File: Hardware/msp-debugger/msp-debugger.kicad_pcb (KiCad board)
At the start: 2 copper layers, 195.6 x 98 mm, 22 parts, among them J1 USB_B_Micro, J2 Conn_02x10, J3 Conn_02x10, J4 Conn_01x04_Pin, SW1 222ADVBA, SW2 222ADVBA, SW3 222ADVBA, SW4 222ADVBA, SW5 222ADVBA, U1 MSP430G2553IN20, U3 BA033CC0FP-E2, U4 FT230XS-R

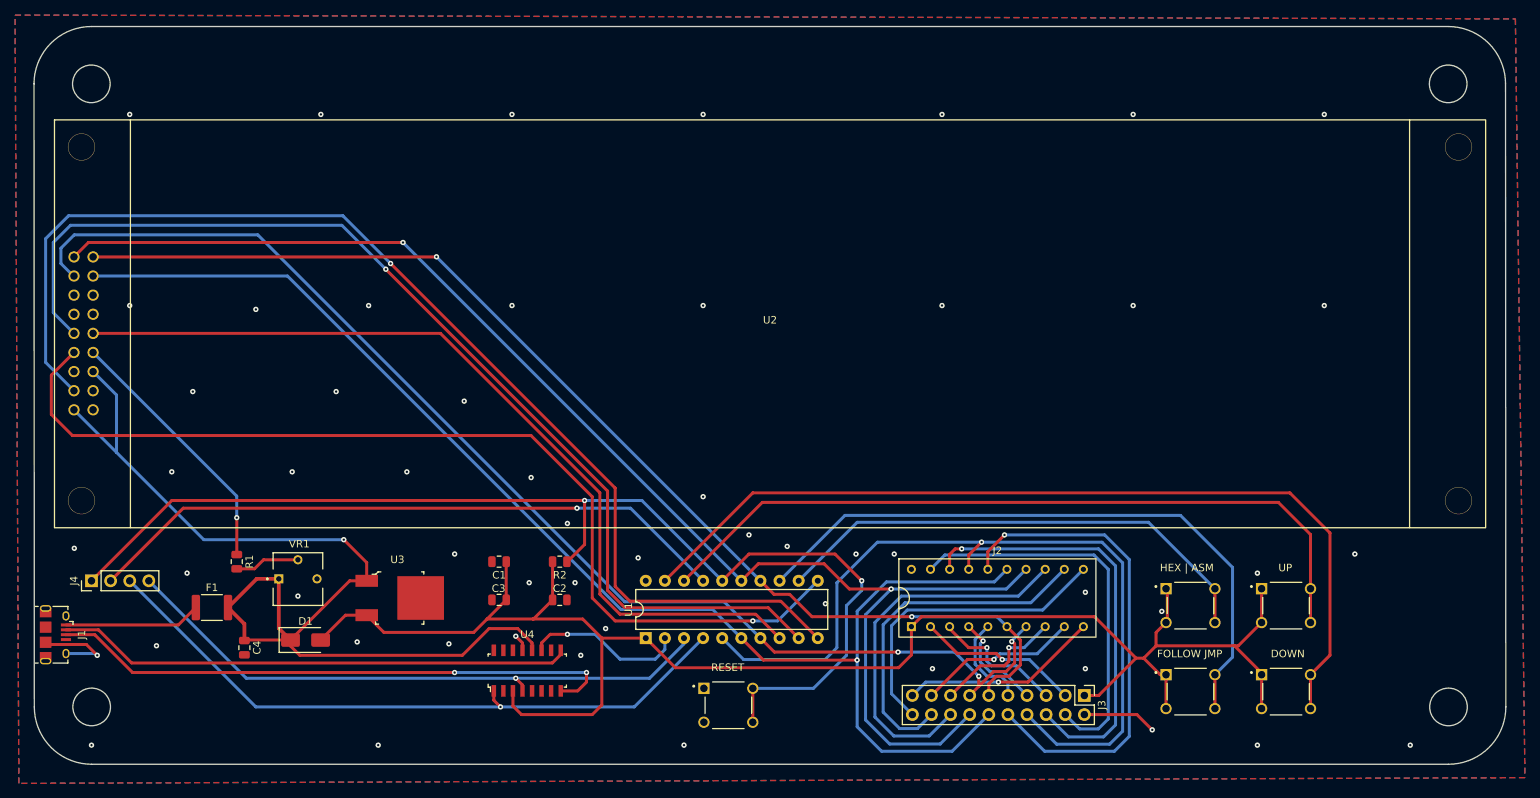
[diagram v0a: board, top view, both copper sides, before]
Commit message: fix hardware issues and route small pcb
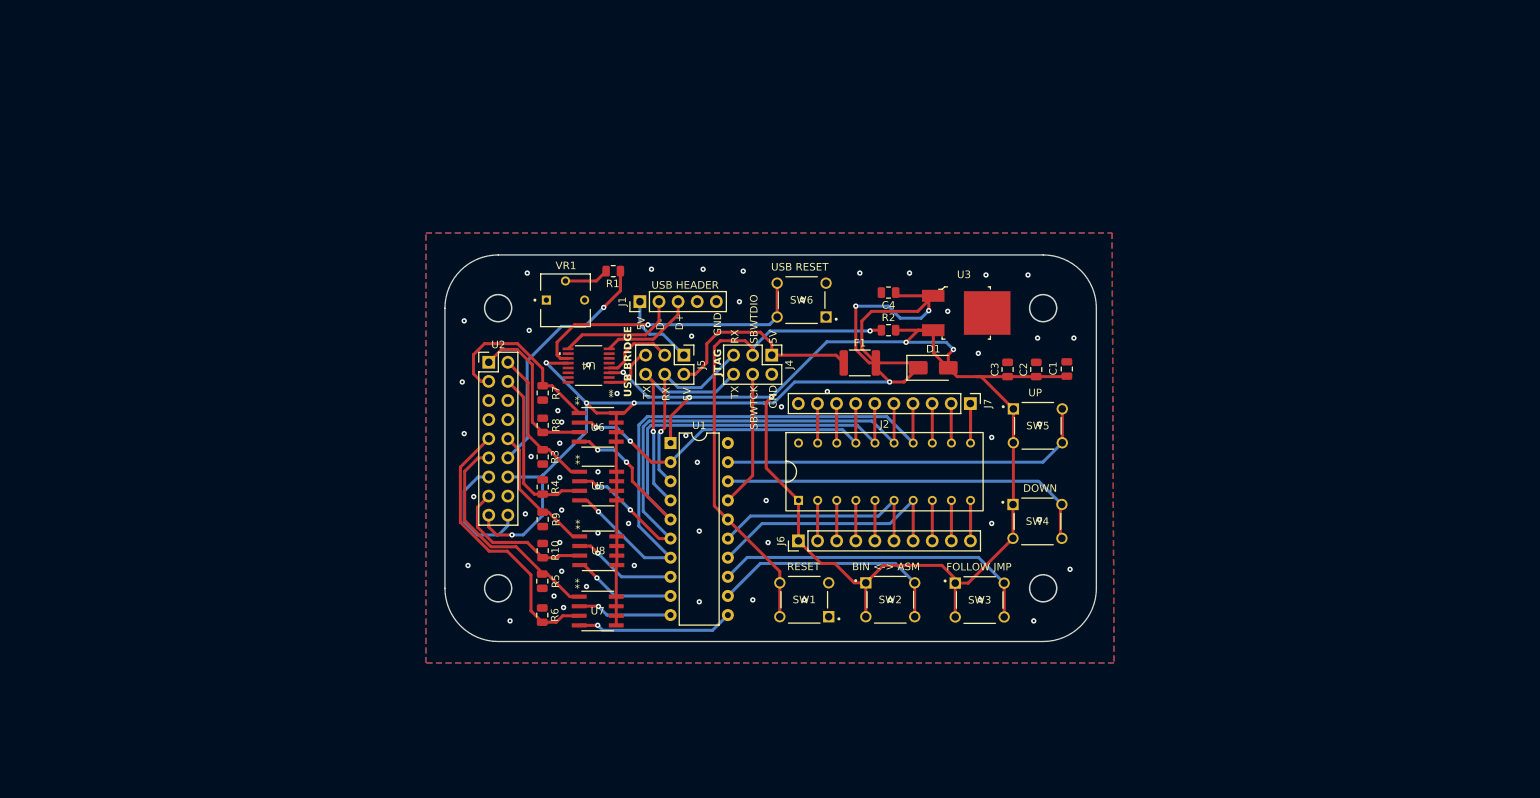
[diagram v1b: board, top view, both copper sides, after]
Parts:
- removed J3: Conn_02x10, Connector_PinHeader_2.54mm:PinHeader_2x10_P2.54mm_Vertical
- added J5: USB JUMPER, Connector_PinHeader_2.54mm:PinHeader_2x03_P2.54mm_Vertical, F.Cu at (137.1, 82.8)
- added J6: Conn_01x10, Connector_PinHeader_2.54mm:PinHeader_1x10_P2.54mm_Vertical, F.Cu at (152.4, 107.5)
- added J7: Conn_01x10, Connector_PinHeader_2.54mm:PinHeader_1x10_P2.54mm_Vertical, F.Cu at (175.2, 89.2)
- added R10: 10K, Capacitor_SMD:C_0805_2012Metric, F.Cu at (118.4, 108.8)
- added R3: 10K, Capacitor_SMD:C_0805_2012Metric, F.Cu at (118.4, 96.3)
- added R4: 10K, Capacitor_SMD:C_0805_2012Metric, F.Cu at (118.4, 100.3)
- added R5: 10K, Capacitor_SMD:C_0805_2012Metric, F.Cu at (118.3, 112.8)
- added R6: 10K, Capacitor_SMD:C_0805_2012Metric, F.Cu at (118.3, 117.3)
- added R7: 10K, Capacitor_SMD:C_0805_2012Metric, F.Cu at (118.4, 87.8)
- added R8: 10K, Capacitor_SMD:C_0805_2012Metric, F.Cu at (118.4, 92.1)
- added R9: 10K, Capacitor_SMD:C_0805_2012Metric, F.Cu at (118.4, 104.6)
- added SW6: 222ADVBA, buttons:SW_222ADVBA, F.Cu at (152.8, 75.5)
- added U5: AO4882, project:SO-8_AOS, F.Cu at (125.7, 100.2)
- added U6: AO4882, project:SO-8_AOS, F.Cu at (125.7, 92.4)
- added U7: AO4882, project:SO-8_AOS, F.Cu at (125.7, 116.8)
- added U8: AO4882, project:SO-8_AOS, F.Cu at (125.8, 108.8)
- J1: footprint Connector_USB:USB_Micro-B_Amphenol_10118194_Horizontal -> Connector_PinHeader_2.54mm:PinHeader_1x05_P2.54mm_Vertical
- J4: value Conn_01x04_Pin -> MSP_FET PORT; footprint Connector_PinHeader_2.54mm:PinHeader_1x04_P2.54mm_Vertical -> Connector_PinHeader_2.54mm:PinHeader_2x03_P2.54mm_Vertical
- U2: footprint project:NHD-0440AZ-FL-YBW -> Connector_PinHeader_2.54mm:PinHeader_2x09_P2.54mm_Vertical
- U4: footprint digikey-footprints:SOIC-16_W3.90mm -> project:SOIC_30XS-R_FTD
- moved C4 97.7 mm to (164.3, 74.5), turned to 180 degrees
- moved J4 95.3 mm to (148.8, 82.8), turned to -90 degrees
- moved F1 92.0 mm to (160.5, 83.8)
- moved D1 90.9 mm to (170.3, 84.5)
- moved J1 89.4 mm to (131.3, 75.7), turned to 90 degrees
- moved U3 84.3 mm to (174.4, 77.2)
- moved C1 79.7 mm to (188.0, 84.6), turned to -90 degrees
- moved C3 74.2 mm to (180.2, 84.7), turned to 90 degrees
- moved C2 70.3 mm to (184.0, 84.7), turned to 90 degrees
- moved R1 63.2 mm to (127.8, 71.6), turned to 180 degrees
- moved R2 53.4 mm to (164.3, 79.5), turned to 0 degrees
- moved VR1 51.4 mm to (121.4, 75.5)
- moved U4 41.4 mm to (124.5, 84.2), turned to 180 degrees
- moved SW5 40.7 mm to (184.2, 92.2)
- moved SW4 40.0 mm to (184.1, 104.9)
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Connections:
- F1 pad 1: Net-(J1-VBUS) -> /PWR_IN
- J1 pad 1: Net-(J1-VBUS) -> /USB_IN
- J2 pad 14: /DB7 -> /DB4
- J2 pad 15: /DB4 -> /DB6
- J2 pad 16: /RST -> /DB7
- J2 pad 17: /TEST -> /DB5
- J2 pad 6: /DB6 -> /TCK
- J2 pad 7: /DB5 -> /TMS
- J4 pad 1: /CNTL RST -> /PWR_IN
- J4 pad 2: /SBWTCK -> GND
- J4 pad 3: /BC_TX -> /CNTL RST
- J4 pad 4: /BC_RX -> /SBWTCK
- U1 pad 10: /E2 -> /RS
- U1 pad 11: /RS -> /E1
- U1 pad 14: /DB6 -> /TMS
- U1 pad 15: /DB7 -> /TCK
- U1 pad 18: /UP SW -> /DOWN SW
- U1 pad 19: /DOWN SW -> /UP SW
- U1 pad 2: /RESET# -> /DB5
- U1 pad 5: /TEST -> /DB7
- U1 pad 6: /DB4 -> /DB6
- U1 pad 7: /DB5 -> /DB4
- U1 pad 9: /E1 -> /E2
- U2 pad 1: /DB7 -> /DB7_5V
- U2 pad 10: /R/W -> /R/W_5V
- U2 pad 11: /RS -> /RS_5V
- U2 pad 15: /E2 -> /E2_5V
- U2 pad 2: /DB6 -> /DB6_5V
- U2 pad 3: /DB5 -> /DB5_5V
- U2 pad 4: /DB4 -> /DB4_5V
- U2 pad 9: /E1 -> /E1_5V
- U4 pad 1: /BC_TX -> /BRIDGE_TX
- U4 pad 4: /BC_RX -> /BRIDGE_RX
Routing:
- net /E2: track 156.6 -> 13.8 mm
- net /E1: track 143.7 -> 20.9 mm
- net /RS: track 132.8 -> 12.6 mm
- net /DB5: track 166.4 -> 46.7 mm, vias 3 -> 2
- net /DB7: track 184.9 -> 67.4 mm
- net /TEST: track 108.8 -> 0.00 mm, vias 1 -> 0
- net /DB4: track 181.1 -> 78.3 mm
- net /R/W: track 115.9 -> 13.8 mm, vias 0 -> 1
- net /CNTL RST: track 152.8 -> 65.2 mm, vias 2 -> 1
- net /DB6: track 154.4 -> 71.7 mm
- net /DOWN SW: track 119.8 -> 50.2 mm
- net /SBWTCK: track 86.7 -> 18.1 mm, vias 1 -> 0
- net /RST: track 65.9 -> 0.00 mm, vias 1 -> 0
- net /D+: track 76.4 -> 12.8 mm, vias 2 -> 0
- net /BC_TX: track 89.4 -> 31.8 mm
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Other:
- board size 195.6 x 98 mm -> 86.6 x 51.4 mm
- board text added: "5V"
- board text added: "D+"
- board text added: "D-"
- board text added: "GND"
- board text added: "JTAG"
- board text added: "RX"
- board text added: "SBWTCK"
- board text added: "SBWTDIO"
- board text added: "TX"
- board text added: "USB BRIDGE"
- board text added: "USB HEADER"
